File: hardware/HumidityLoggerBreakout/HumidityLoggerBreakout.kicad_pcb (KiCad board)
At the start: 2 copper layers, 98 x 74 mm, 45 parts, among them J1 PWR_IN, J2 BME280, J3 +5V_OUT, J4 IO, J6 Conn_01x11, J7 Conn_01x11, J8 I2C_MCU, U1 LM317_TO-252

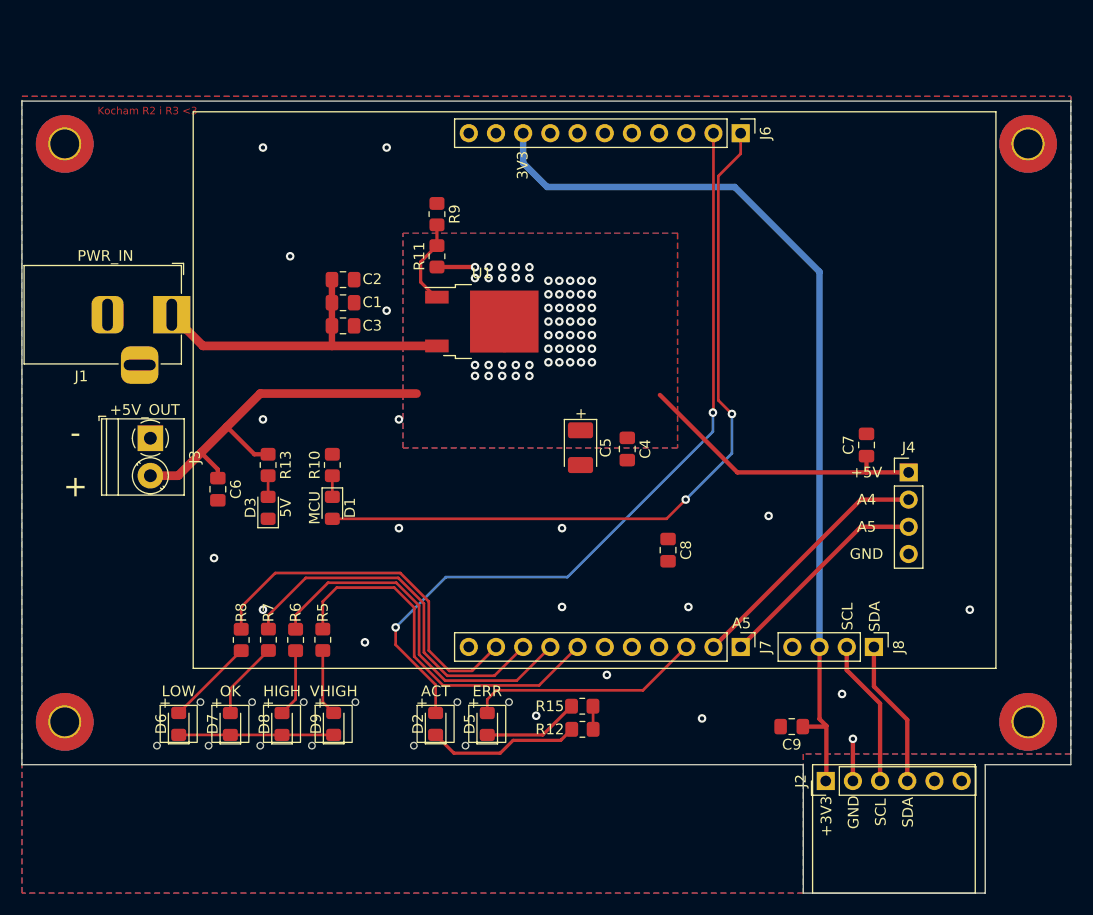
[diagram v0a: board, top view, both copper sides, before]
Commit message: WIP on the board.
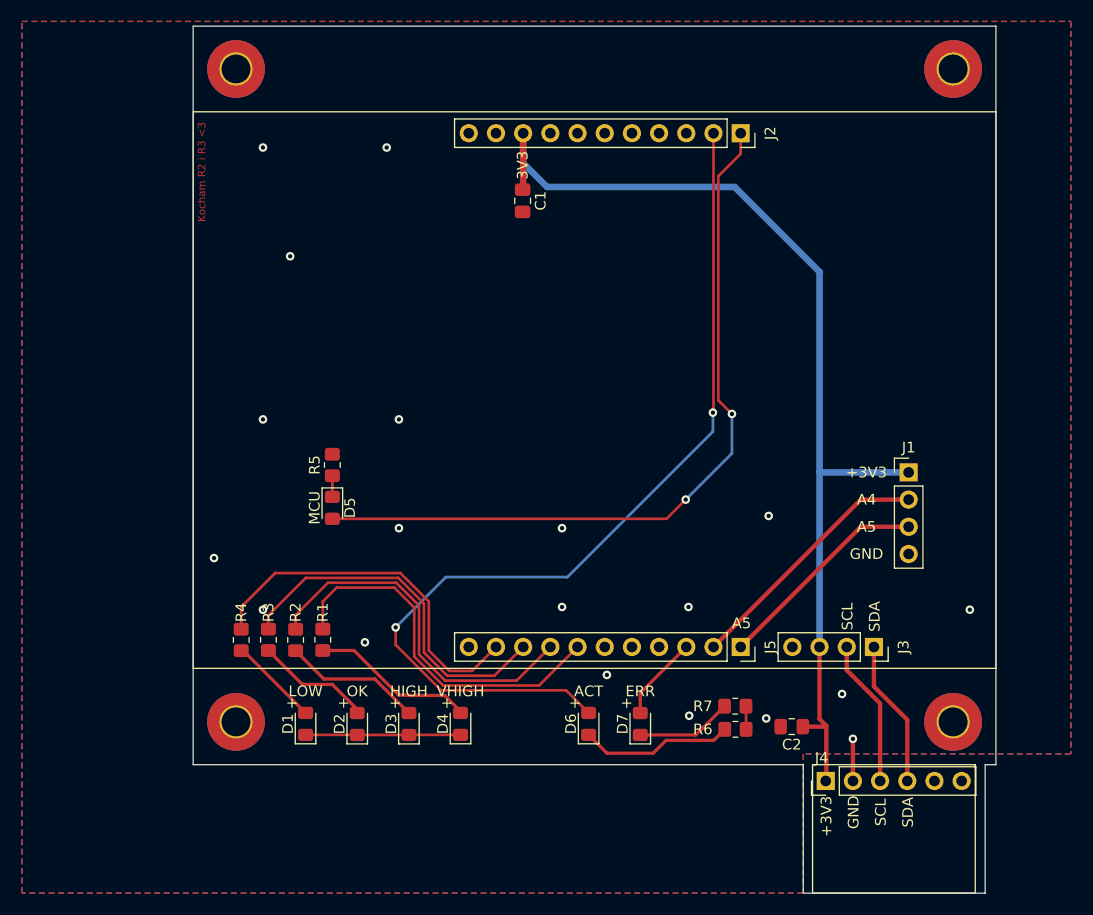
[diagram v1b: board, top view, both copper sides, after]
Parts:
- removed the C2 at (104.0, 65.7)
- removed C3, C4, C6, C7, C8: 100n, Capacitor_SMD:C_0805_2012Metric_Pad1.18x1.45mm_HandSolder
- removed C5: 100u, Capacitor_Tantalum_SMD:CP_EIA-3528-12_Kemet-T_Pad1.50x2.35mm_HandSolder
- removed the D3 at (97.0, 87.0)
- removed the J1 at (88.0, 69.0)
- removed the J3 at (86.0, 80.5)
- removed R11: 330, Resistor_SMD:R_0805_2012Metric_Pad1.20x1.40mm_HandSolder
- removed R13, R9: 1k, Resistor_SMD:R_0805_2012Metric_Pad1.20x1.40mm_HandSolder
- removed REF** (x6): VLP-XXX-X, marcin_library:VLP-XXX-X
- removed U1: LM317_TO-252, Package_TO_SOT_SMD:TO-252-2
- J2: renamed from J6; footprint Connector_PinHeader_2.54mm:PinHeader_1x11_P2.54mm_Vertical -> Connector_PinSocket_2.54mm:PinSocket_1x11_P2.54mm_Vertical
- J3: renamed from J8; footprint Connector_PinHeader_2.54mm:PinHeader_1x04_P2.54mm_Vertical -> Connector_PinSocket_2.54mm:PinSocket_1x04_P2.54mm_Vertical
- J5: renamed from J7; footprint Connector_PinHeader_2.54mm:PinHeader_1x11_P2.54mm_Vertical -> Connector_PinSocket_2.54mm:PinSocket_1x11_P2.54mm_Vertical
- moved C1 19.3 mm to (120.8, 58.3), turned to -90 degrees
- moved H1 17.5 mm to (94.0, 46.0)
- moved H4 16.0 mm to (94.0, 107.0)
- moved D7 14.3 mm to (131.8, 107.2)
- moved D6 14.3 mm to (126.9, 107.2)
- moved R6 14.3 mm to (140.7, 107.7)
- moved R7 14.3 mm to (140.6, 105.5)
- moved D1 11.9 mm to (100.5, 107.2)
- moved D2 11.9 mm to (105.3, 107.2)
- moved D3 11.9 mm to (110.2, 107.2)
- moved D4 11.9 mm to (115.0, 107.2)
- moved H2 9.90 mm to (161.0, 46.0)
- moved H3 7.00 mm to (161.0, 107.0)
- renumbered C9 to C2, D6 to D1, D7 to D2, D8 to D3, D9 to D4, D1 to D5, D2 to D6, D5 to D7, J4 to J1, J2 to J4, R5 to R1, R6 to R2, R7 to R3, R8 to R4, R10 to R5, R12 to R6, R15 to R7
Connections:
- C1 pad 1: +12V -> +3.3V
- J1 pad 1: +5V -> +3.3V
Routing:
- net +5V: track 69.8 -> 0.00 mm, vias 55 -> 0
- net +12V: track 32.2 -> 0.00 mm
- net /A3: track 21.9 -> 7.95 mm
- net +3.3V: track 84.7 -> 98.4 mm
- net /D3: track 74.7 -> 87.4 mm
- net Net-(D4-Pad2): track 6.25 -> 15.4 mm
- net Net-(R11-Pad2): track 7.97 -> 0.00 mm
- net Net-(D3-Pad2): track 6.35 -> 13.0 mm
- net Net-(D2-Pad2): track 7.31 -> 10.9 mm
- net Net-(D3-Pad2) (its old number): track 1.97 -> 0.00 mm
- net Net-(D7-Pad1): track 9.73 -> 8.99 mm
- net GND: track 20.8 -> 20.6 mm, vias 20 -> 19
- removed copper zone on B.Cu, net +5V
- removed copper zone on F.Cu, net +5V
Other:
- board size 98 x 74 mm -> 75 x 81 mm
- board text removed: "+5V"
- board text removed: "-"
